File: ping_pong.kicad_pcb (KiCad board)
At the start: 2 copper layers, 100 x 80 mm, 48 parts, among them J101 5V_IN, J102 12V_IN, J103 GND_IN, J104 STEPPER_OUT1, J105 ENABLE, J106 STEP1, J107 DIR1, J109 STEP2, J110 DIR2, J111 STEPPER_OUT2, J113 STEP3, J114 DIR3, J115 STEPPER_OUT3, J117 STEP4, J118 DIR4, J119 STEPPER_OUT4, J120 6V_for_Hbridge, J121 5V_for_ultrasonic1, J122 5V_for_ultrasonic2, J123 5V_for_ultrasonic3, J124 5V_for_ultrasonic4, J125 GND_for_ultrasonic1, J126 GND_for_ultrasonic2, J127 GND_for_ultrasonic3, J128 GND_for_ultrasonic4, J129 5V_for_pixycam, J130 GND_for_Hbridge, J131 3.3V_IN, J132 GND_for_xbee, J133 GND_for_pixycam, J134 GND_backup1, J135 GND_backup2, J138 5V_backup1, J139 5V_backup2, J140 5V_backup3, J141 5V_backup4, J142 3.3V_for_xbee, J143 3.3V_backup1, J144 3.3V_backup2, J145 5V_SERVO1, J146 5V_SERVO2, J147 GND_SERVO1, J148 GND_SERVO1

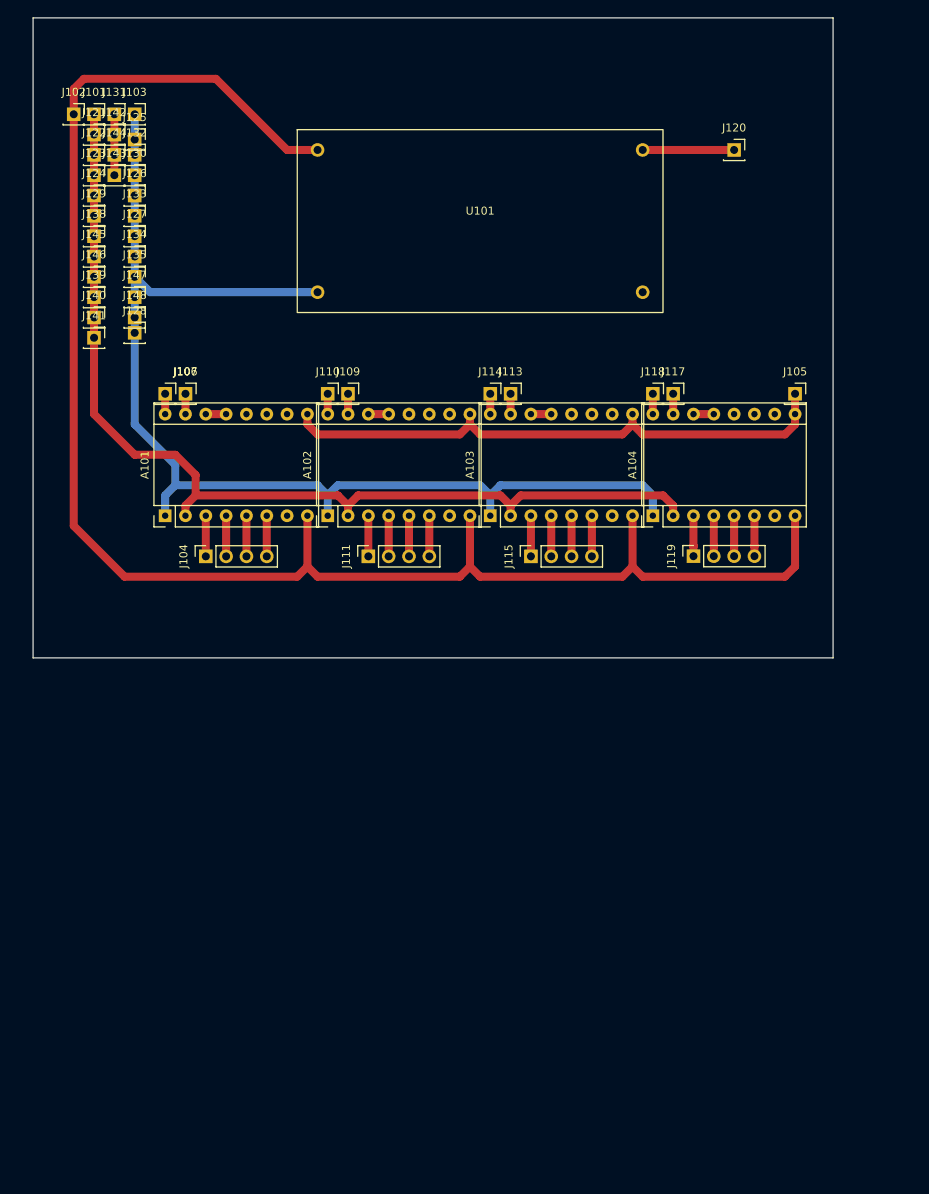
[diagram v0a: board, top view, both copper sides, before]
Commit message: checkpoint
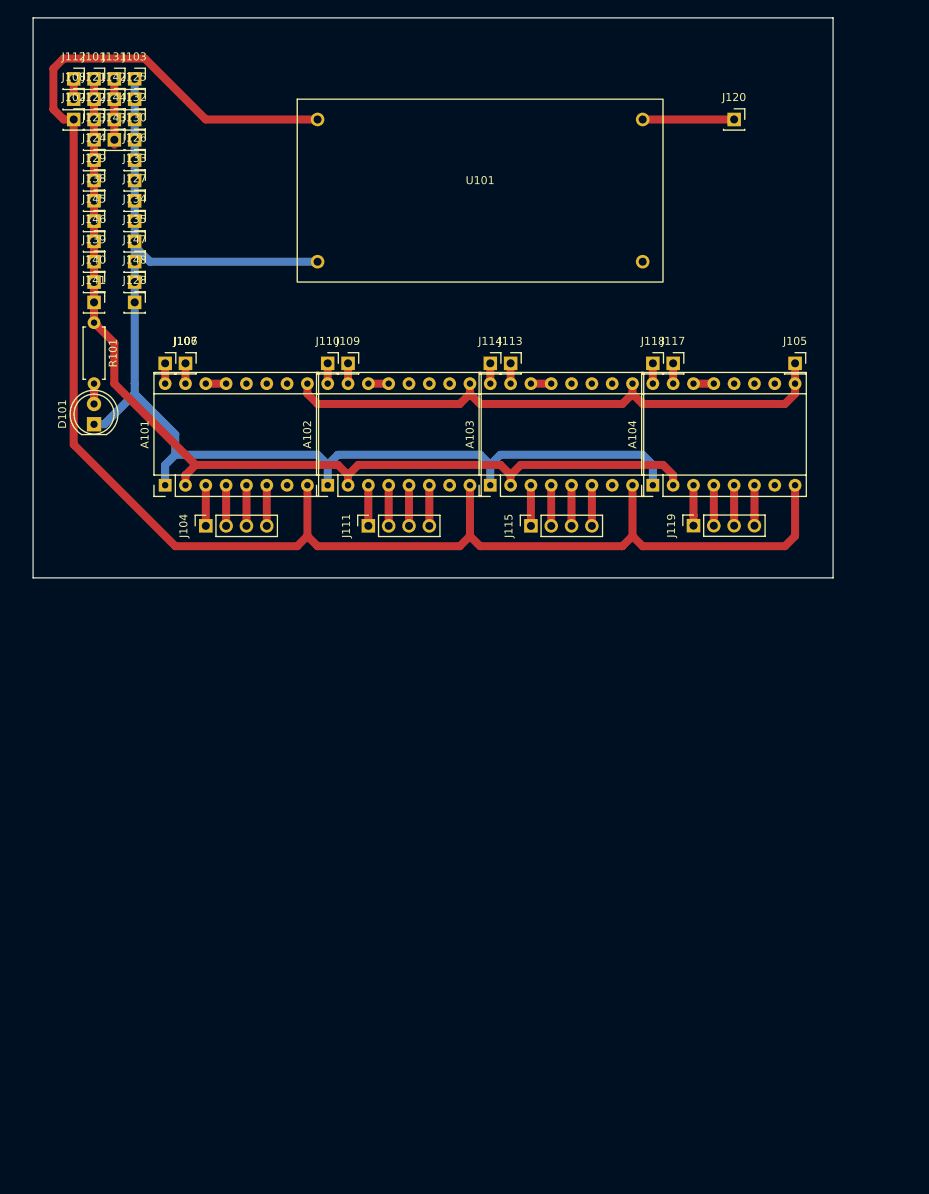
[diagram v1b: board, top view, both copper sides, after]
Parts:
- added D101: LED, MyLED:LED_D5.0mm, F.Cu at (7.62, 49.5)
- added J108: AMMETER+, MyPinSocket:MyPinSocket, F.Cu at (5.08, 10.2)
- added J112: 12V_IN, MyPinSocket:MyPinSocket, F.Cu at (5.08, 7.62)
- added R101: R, My7.62mmResistor:My7.62mmResistor, F.Cu at (7.62, 38.1)
- J102: value 12V_IN -> AMMETER-
- moved J125 5.04 mm to (12.7, 10.2)
- moved J122 4.43 mm to (7.62, 12.7)
- moved J127 4.43 mm to (12.7, 22.9)
- moved J132 4.43 mm to (12.7, 12.7)
- moved J134 4.43 mm to (12.7, 25.4)
- moved J138 4.43 mm to (7.62, 22.9)
- moved J144 4.43 mm to (10.2, 12.7)
- moved J145 4.43 mm to (7.62, 25.4)
- moved J121 4.43 mm to (7.62, 10.2)
- moved J123 4.43 mm to (7.62, 15.2)
- moved J130 4.43 mm to (12.7, 15.2)
- moved J142 4.43 mm to (10.2, 10.2)
- moved J143 4.43 mm to (10.2, 15.2)
- moved J101 4.43 mm to (7.62, 7.62)
- moved J103 4.43 mm to (12.7, 7.62)
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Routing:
- net GND: track 146.4 -> 153.1 mm
- net Net-(J108-Pin_1): track 0.00 -> 2.54 mm
- net Net-(D101-A): track 0.00 -> 2.54 mm
- net 5V: track 125.1 -> 122.7 mm
- net 12V: track 211.2 -> 210.0 mm
- net 3.3V: track 7.62 -> 8.24 mm
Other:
- board size 100 x 80 mm -> 100 x 70 mm

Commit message: checkpoint
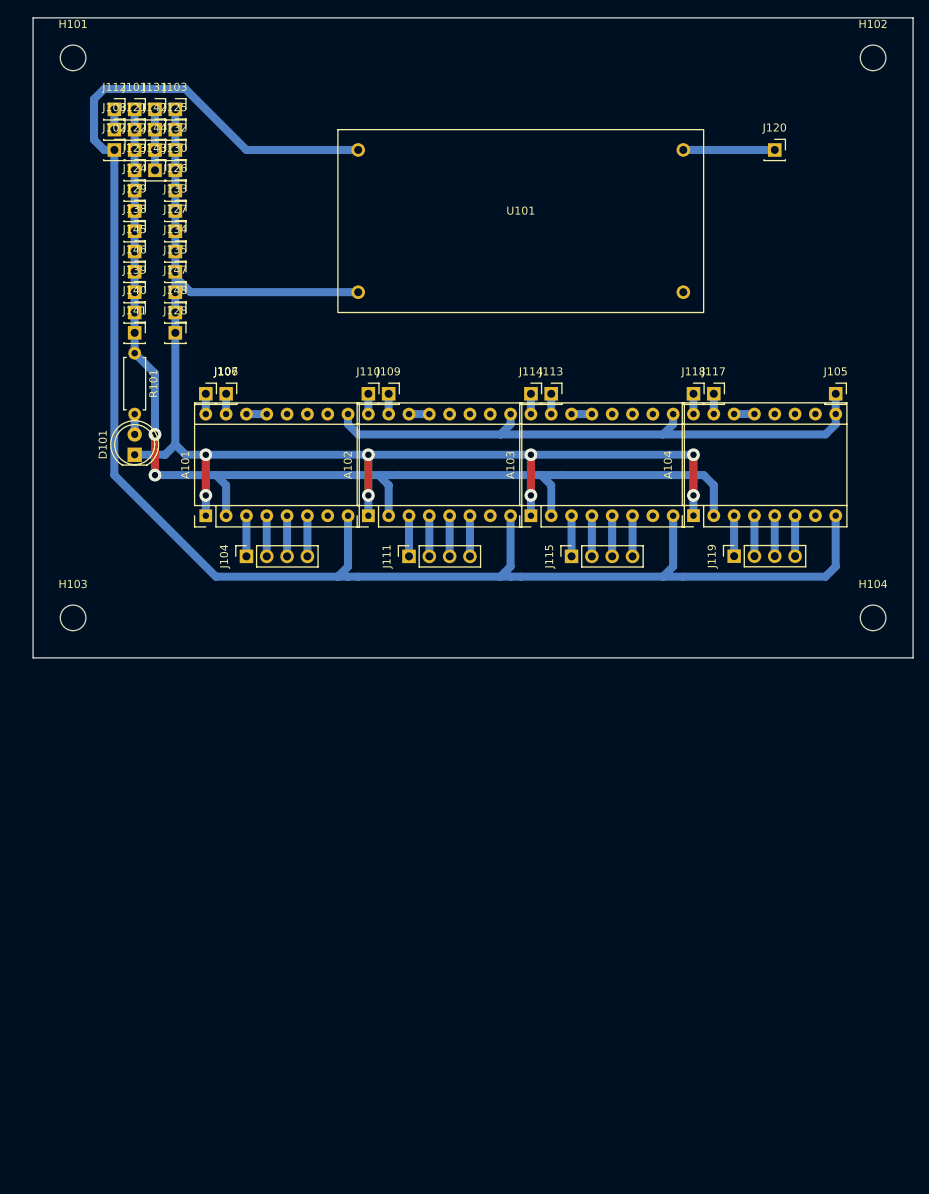
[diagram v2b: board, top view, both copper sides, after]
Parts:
- added H101: MountingHole, MountingHole:MountingHole_3.2mm_M3, F.Cu at (5.00, 5.00)
- added H102: MountingHole, MountingHole:MountingHole_3.2mm_M3, F.Cu at (105.0, 5.00)
- added H103: MountingHole, MountingHole:MountingHole_3.2mm_M3, F.Cu at (5.00, 75.0)
- added H104: MountingHole, MountingHole:MountingHole_3.2mm_M3, F.Cu at (105.0, 75.0)
- moved J109 6.35 mm to (44.5, 47.0)
- moved J111 6.35 mm to (47.0, 67.3)
- moved J115 6.35 mm to (67.3, 67.3)
- moved J104 6.35 mm to (26.7, 67.3)
- moved J127 6.35 mm to (17.8, 26.7)
- moved J132 6.35 mm to (17.8, 16.5)
- moved J134 6.35 mm to (17.8, 29.2)
- moved D101 6.35 mm to (12.7, 53.3)
- moved J102 6.35 mm to (10.2, 16.5)
- moved J103 6.35 mm to (17.8, 11.4)
- moved J122 6.35 mm to (12.7, 16.5)
- moved J125 6.35 mm to (17.8, 14.0)
- moved J130 6.35 mm to (17.8, 19.1)
- moved J138 6.35 mm to (12.7, 26.7)
- moved J144 6.35 mm to (15.2, 16.5)
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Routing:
- net 5V: track 122.7 -> 137.8 mm, vias 0 -> 2
- net GND: track 153.1 -> 166.3 mm, vias 0 -> 8
- net 12V: track 210.0 -> 212.2 mm
- net ENABLE: track 71.7 -> 73.2 mm
- net 3.3V: track 8.24 -> 7.62 mm
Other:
- board size 100 x 70 mm -> 110 x 80 mm

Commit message: checkpoint
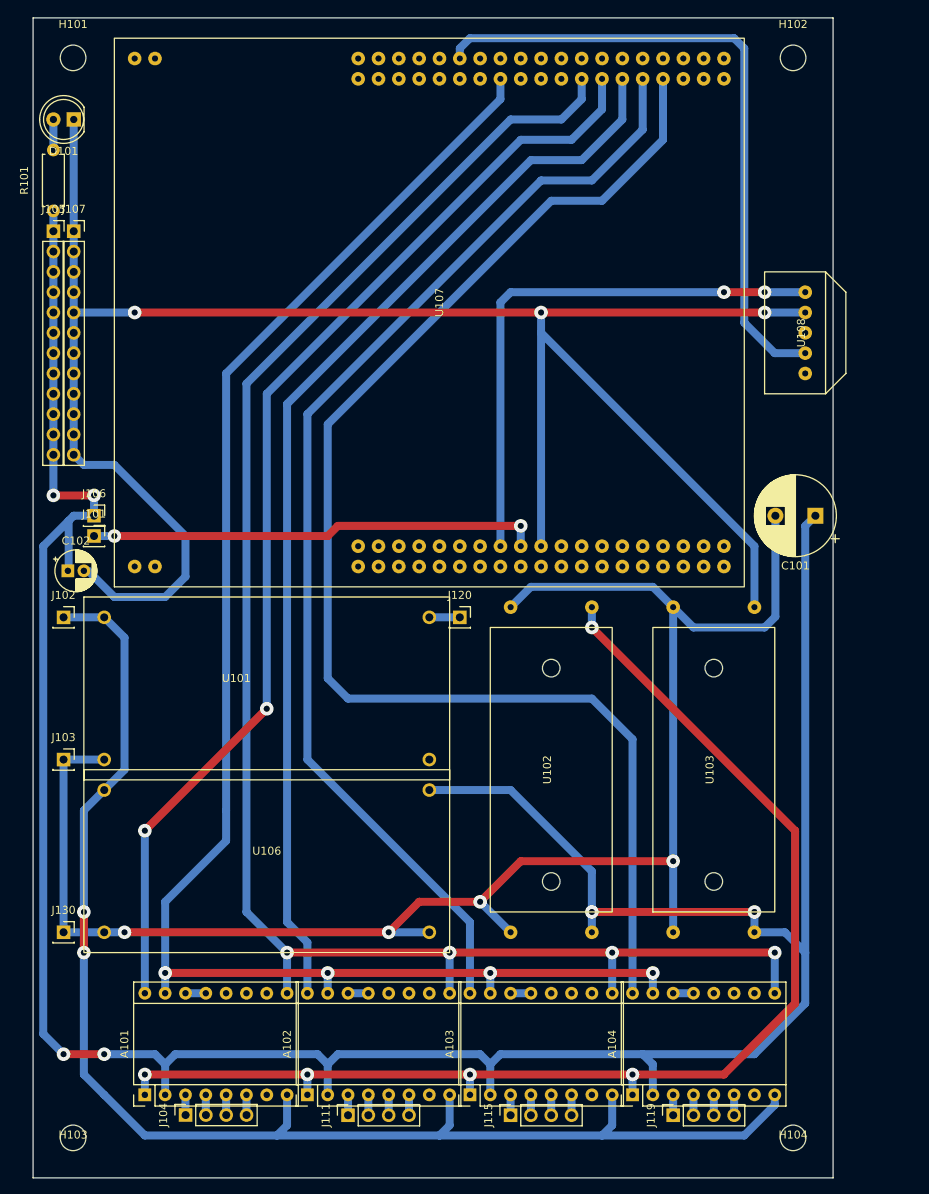
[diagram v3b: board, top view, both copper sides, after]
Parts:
- removed J108: AMMETER+, MyPinSocket:MyPinSocket
- removed J109: STEP2, MyPinSocket:MyPinSocket
- removed J110: DIR2, MyPinSocket:MyPinSocket
- removed J112: 12V_IN, MyPinSocket:MyPinSocket
- removed J113: STEP3, MyPinSocket:MyPinSocket
- removed J114: DIR3, MyPinSocket:MyPinSocket
- removed J117: STEP4, MyPinSocket:MyPinSocket
- removed J118: DIR4, MyPinSocket:MyPinSocket
- removed J121: 5V_for_ultrasonic1, MyPinSocket:MyPinSocket
- removed J122: 5V_for_ultrasonic2, MyPinSocket:MyPinSocket
- removed J123: 5V_for_ultrasonic3, MyPinSocket:MyPinSocket
- removed J124: 5V_for_ultrasonic4, MyPinSocket:MyPinSocket
- removed J125: GND_for_ultrasonic1, MyPinSocket:MyPinSocket
- removed J126: GND_for_ultrasonic2, MyPinSocket:MyPinSocket
- removed J127: GND_for_ultrasonic3, MyPinSocket:MyPinSocket
- removed J128: GND_for_ultrasonic4, MyPinSocket:MyPinSocket
- removed J129: 5V_for_pixycam, MyPinSocket:MyPinSocket
- removed J131: 3.3V_IN, MyPinSocket:MyPinSocket
- removed J132: GND_for_xbee, MyPinSocket:MyPinSocket
- removed J133: GND_for_pixycam, MyPinSocket:MyPinSocket
- removed J134: GND_backup1, MyPinSocket:MyPinSocket
- removed J135: GND_backup2, MyPinSocket:MyPinSocket
- removed J138: 5V_backup1, MyPinSocket:MyPinSocket
- removed J139: 5V_backup2, MyPinSocket:MyPinSocket
- removed J140: 5V_backup3, MyPinSocket:MyPinSocket
- removed J141: 5V_backup4, MyPinSocket:MyPinSocket
- removed J142: 3.3V_for_xbee, MyPinSocket:MyPinSocket
- removed J143: 3.3V_backup1, MyPinSocket:MyPinSocket
- removed J144: 3.3V_backup2, MyPinSocket:MyPinSocket
- removed J145: 5V_SERVO1, MyPinSocket:MyPinSocket
- removed J146: 5V_SERVO2, MyPinSocket:MyPinSocket
- removed J147, J148: GND_SERVO1, MyPinSocket:MyPinSocket
- added C101: 1000u, Capacitor_THT:CP_Radial_D10.0mm_P5.00mm, F.Cu at (97.8, 62.2)
- added C102: 10u, Capacitor_THT:CP_Radial_D5.0mm_P2.00mm, F.Cu at (4.35, 69.1)
- added U102: ~, Ammeter:Ammeter, F.Cu at (64.8, 94.0)
- added U103: ~, Ammeter:Ammeter, F.Cu at (85.1, 94.0)
- added U106: 5V_OUT, LM2596:LM2596, F.Cu at (29.2, 106.7)
- added U107: ~, NUCLEO-F401RE:NUCLEO-F401RE, F.Cu at (50.8, 35.6)
- added U108: ~, XBEE:XBEE, F.Cu at (96.5, 39.4)
- J101: value 5V_IN -> 5V_OPTIONAL-
- J102: value AMMETER- -> 12V_IN
- J105: value ENABLE -> 5V_Sockets; footprint MyPinSocket:MyPinSocket -> Connector_PinSocket_2.54mm:PinSocket_1x12_P2.54mm_Vertical
- J106: value STEP1 -> 5V_OPTIONAL+
- J107: value DIR1 -> 5V_GND_Sockets; footprint MyPinSocket:MyPinSocket -> Connector_PinSocket_2.54mm:PinSocket_1x12_P2.54mm_Vertical
- U101: value ~ -> 6V_OUT
- moved J105 99.9 mm to (2.54, 26.7)
- moved J130 96.3 mm to (3.81, 114.3)
- moved J103 82.5 mm to (3.81, 92.7)
- moved A104 72.8 mm to (74.9, 134.6)
- moved A101 72.8 mm to (14.0, 134.6)
- moved A102 72.8 mm to (34.3, 134.6)
- moved A103 72.8 mm to (54.6, 134.6)
- moved J120 70.4 mm to (53.3, 74.9)
- moved J119 70.3 mm to (80.0, 137.2)
- moved J111 70.3 mm to (39.4, 137.2)
- moved J115 70.3 mm to (59.7, 137.2)
- moved J104 70.2 mm to (19.1, 137.1)
- moved U101 66.5 mm to (29.2, 85.1)
- moved H104 65.8 mm to (95.0, 140.0)
- moved H103 65.0 mm to (5.00, 140.0)
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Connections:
- A101 pad 1: GND -> 12V_GND
- A101 pad 15: Net-(A101-STEP) -> STEP
- A101 pad 16: Net-(A101-DIR) -> DIR1
- A102 pad 1: GND -> 12V_GND
- A102 pad 15: Net-(A102-STEP) -> STEP
- A102 pad 16: Net-(A102-DIR) -> DIR2
- A103 pad 1: GND -> 12V_GND
- A103 pad 15: Net-(A103-STEP) -> STEP
- A103 pad 16: Net-(A103-DIR) -> DIR3
- A104 pad 1: GND -> 12V_GND
- A104 pad 15: Net-(A104-STEP) -> STEP
- A104 pad 16: Net-(A104-DIR) -> DIR4
- D101 pad 1: GND -> 5V_GND
- J101 pad 1: 5V -> Net-(J101-Pin_1)
- J105 pad 1: ENABLE -> 5V
- J106 pad 1: Net-(A101-STEP) -> 5V
- J107 pad 1: Net-(A101-DIR) -> 5V_GND
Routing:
- net 5V_GND: track 0.00 -> 246.3 mm, vias 0 -> 3
- net 5V: track 137.8 -> 361.4 mm, vias 2 -> 6
- net STEP: track 0.00 -> 200.2 mm, vias 0 -> 4
- net DIR4: track 0.00 -> 169.0 mm
- net 12V_GND: track 0.00 -> 155.2 mm, vias 0 -> 5
- net DIR3: track 0.00 -> 143.8 mm
- net DIR1: track 0.00 -> 141.7 mm, vias 0 -> 2
- net ENABLE: track 73.2 -> 213.7 mm, vias 0 -> 4
- net DIR2: track 0.00 -> 136.4 mm
- net RX: track 0.00 -> 81.4 mm
- net 3V3: track 0.00 -> 69.1 mm, vias 0 -> 2
- net Net-(J101-Pin_1): track 0.00 -> 56.4 mm, vias 0 -> 2
- net GND: track 166.3 -> 207.1 mm, vias 8 -> 4
- net 12V: track 212.2 -> 174.6 mm, vias 0 -> 2
- net 3.3V: track 7.62 -> 0.00 mm
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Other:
- board size 110 x 80 mm -> 100 x 145 mm
